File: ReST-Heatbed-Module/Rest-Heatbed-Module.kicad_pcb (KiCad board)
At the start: 2 copper layers, 31 x 49.2 mm, 72 parts

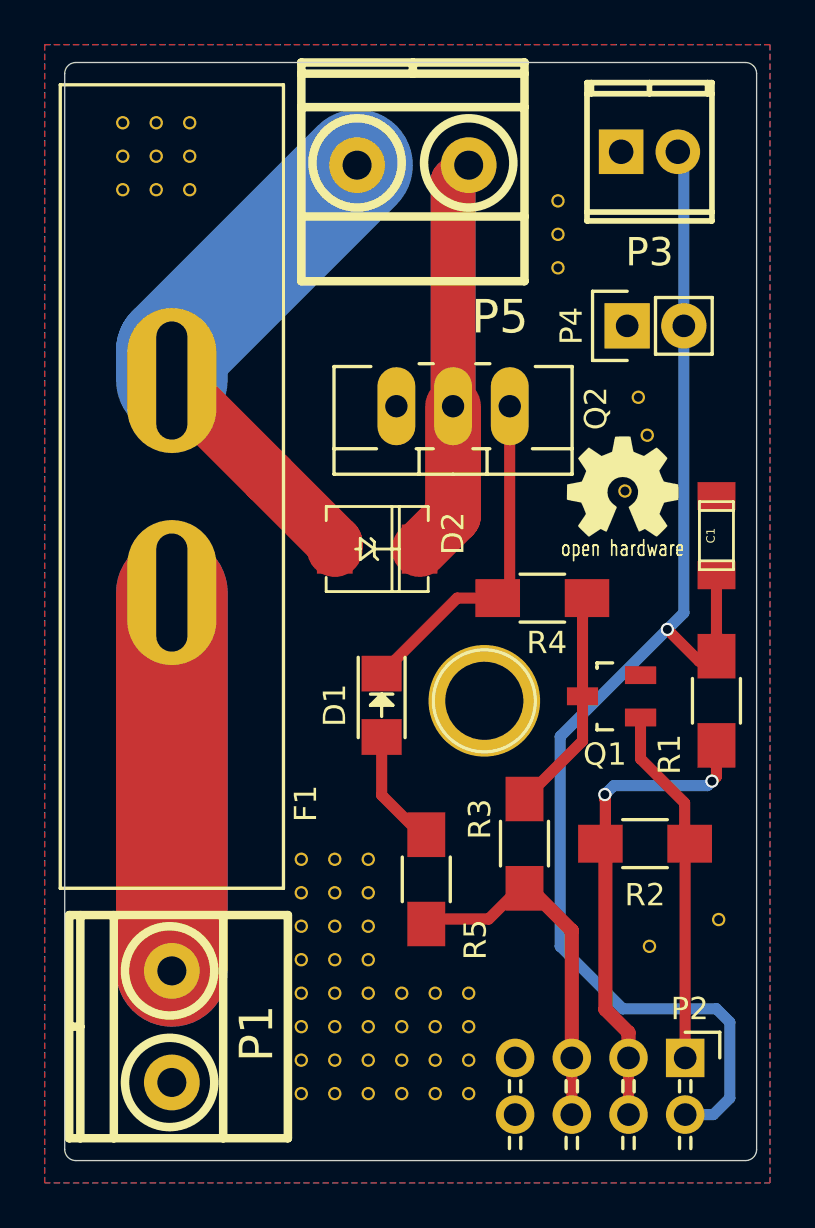
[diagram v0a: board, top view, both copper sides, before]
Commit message: Final release
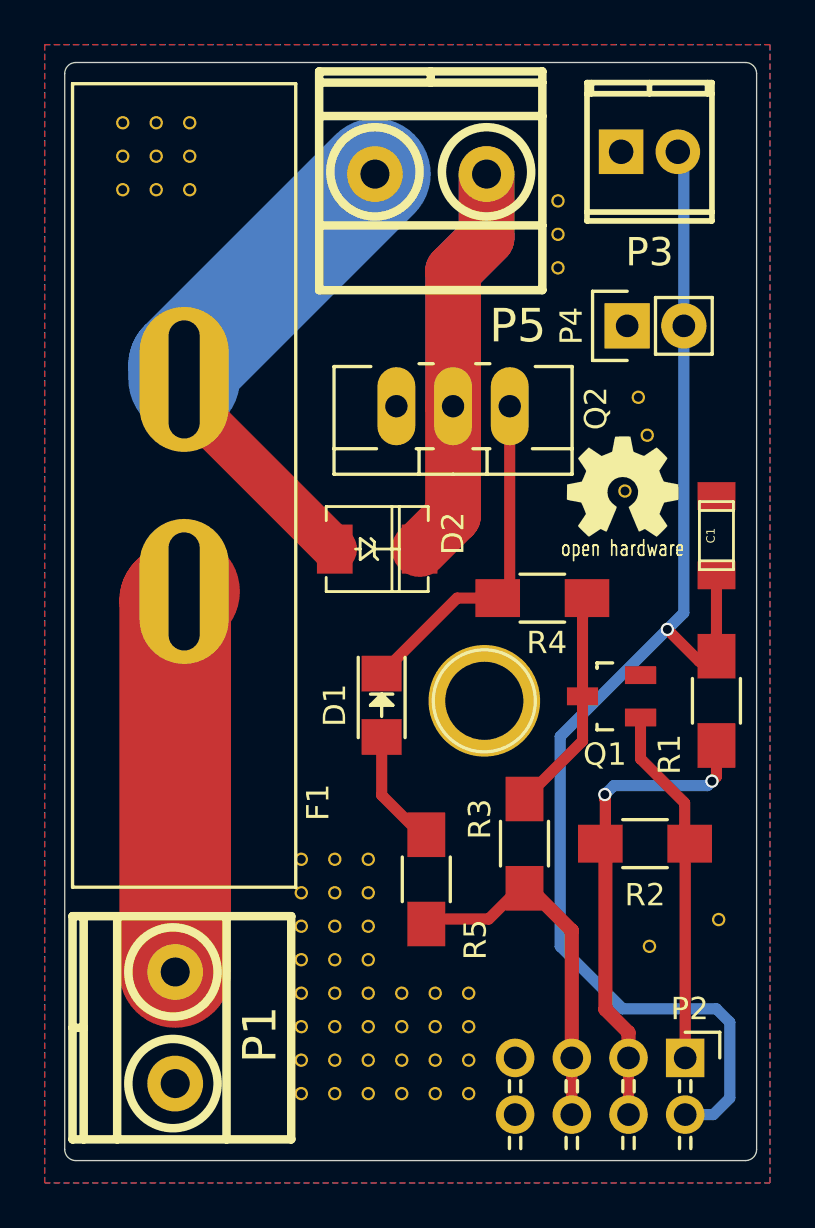
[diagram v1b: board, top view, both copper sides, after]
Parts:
- moved P5 0.89 mm to (128.6, 110.4)
- moved F1 0.55 mm to (117.5, 124.3)
- moved P1 0.16 mm to (117.2, 148.7)
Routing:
- net Net-(F1-Pad1): track 33.9 -> 17.2 mm
- net +12V: track 23.7 -> 23.1 mm
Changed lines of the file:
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@@
     (links 82)
     (no_connects 0)
-    (area 109.4 102.4 144.075 163.425001)
+    (area 109.55 102.8 144.075 156.075)
     (thickness 1.6)
     (drawings 10)
-    (tracks 69)
+    (tracks 70)
     (zones 0)
     (modules 72)
@@
     (visible_elements 7FFFFFFF)
     (pcbplotparams
-      (layerselection 0x00030_80000001)
-      (usegerberextensions false)
+      (layerselection 0x010f0_80000001)
+      (usegerberextensions true)
       (excludeedgelayer true)
       (linewidth 0.100000)
@@
       (outputformat 1)
       (mirror false)
-      (drillshape 1)
+      (drillshape 0)
       (scaleselection 1)
-      (outputdirectory ""))
+      (outputdirectory ../Gerber/Heatbed/))
   )
   (net 0 "")
@@
   )
   (module ReST-Librar:JEF-703C (layer F.Cu)
-    (at 117 124.4 90)
+    (at 117.55 124.35 90)
     (fp_text reference F1 (at -14.2 6 90) (layer F.SilkS)
       (effects (font (size 1 1) (thickness 0.15)))
@@
   )
   (module 5mm-pitch-terminal:mkds_1,5-2 (layer F.Cu)
-    (at 117 148.6 270)
+    (at 117.15 148.65 270)
     (descr "2-way 5mm pitch terminal block, Phoenix MKDS series")
     (fp_text reference P1 (at 0.3 -3.8 270) (layer F.SilkS)
@@
   )
   (module 5mm-pitch-terminal:mkds_1,5-2 (layer F.Cu)
-    (at 127.8 110 180)
+    (at 128.6 110.4 180)
     (descr "2-way 5mm pitch terminal block, Phoenix MKDS series")
     (fp_text reference P5 (at -3.9 -6.8 180) (layer F.SilkS)
@@
   (segment (start 131.6 129.4) (end 132.14 128.86) (width 0.5) (layer F.Cu) (net 4))
   (segment (start 132.14 128.86) (end 132.14 120.8) (width 0.5) (layer F.Cu) (net 4))
-  (segment (start 124.30008 127.2) (end 124.30008 126.95008) (width 2.5) (layer F.Cu) (net 5))
-  (segment (start 124.30008 126.95008) (end 121.35 124) (width 2.5) (layer F.Cu) (net 5))
-  (segment (start 121.35 124) (end 117 119.65) (width 2.5) (layer F.Cu) (net 5))
-  (segment (start 117 119.65) (end 117 118.3) (width 5) (layer B.Cu) (net 5))
-  (segment (start 117 118.3) (end 125.3 110) (width 5) (layer B.Cu) (net 5))
+  (segment (start 124.30008 127.2) (end 117.55 120.44992) (width 2) (layer F.Cu) (net 5))
+  (segment (start 117.55 120.44992) (end 117.55 119.6) (width 2) (layer F.Cu) (net 5))
+  (segment (start 126.1 110.4) (end 117.55 118.95) (width 5) (layer B.Cu) (net 5))
+  (segment (start 117.55 118.95) (end 117.55 119.6) (width 5) (layer B.Cu) (net 5))
+  (segment (start 129.6 120.8) (end 129.6 114.75) (width 2.5) (layer B.Cu) (net 6))
+  (segment (start 129.6 114.75) (end 131.1 113.25) (width 2.5) (layer B.Cu) (net 6))
+  (segment (start 131.1 113.25) (end 131.1 110.4) (width 2.5) (layer B.Cu) (net 6))
+  (segment (start 129.6 120.8) (end 129.6 114.75) (width 2.5) (layer F.Cu) (net 6))
+  (segment (start 129.6 114.75) (end 131.1 113.25) (width 2.5) (layer F.Cu) (net 6))
+  (segment (start 131.1 113.25) (end 131.1 110.4) (width 2.5) (layer F.Cu) (net 6))
   (segment (start 128.09992 127.2) (end 129.6 125.69992) (width 2.5) (layer F.Cu) (net 6))
   (segment (start 129.6 125.69992) (end 129.6 120.8) (width 2.5) (layer F.Cu) (net 6))
-  (segment (start 129.6 120.8) (end 129.6 110.7) (width 2) (layer B.Cu) (net 6) (status 10))
-  (segment (start 129.6 110.7) (end 130.3 110) (width 2) (layer B.Cu) (net 6))
-  (segment (start 129.6 120.8) (end 129.6 110.7) (width 2) (layer F.Cu) (net 6) (status 10))
-  (segment (start 129.6 110.7) (end 130.3 110) (width 2) (layer F.Cu) (net 6))
-  (segment (start 117 129.15) (end 117 146.1) (width 5) (layer B.Cu) (net 7))
-  (segment (start 117 146.1) (end 117 129.15) (width 5) (layer F.Cu) (net 7))
+  (segment (start 117.15 146.15) (end 117.15 129.5) (width 5) (layer F.Cu) (net 7))
+  (segment (start 117.15 129.5) (end 117.55 129.1) (width 5) (layer F.Cu) (net 7))
   (segment (start 134.92 152.54) (end 134.92 150) (width 0.5) (layer F.Cu) (net 8))
   (segment (start 128.4 143.77546) (end 131.2 143.77546) (width 0.5) (layer F.Cu) (net 8))
